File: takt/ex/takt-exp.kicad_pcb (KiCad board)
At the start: 2 copper layers, 40.3 x 128.5 mm, 55 parts, among them J1 PJ301M-12, J2 PJ301M-12, J3 PJ301M-12, J4 PJ301M-12, J5 PJ301M-12, J6 PJ301M-12, J7 PJ301M-12, J8 PJ301M-12, J9 PJ301M-12, Q1 2N3904, Q2 2N3904, Q3 2N3904, SW1 SW_SP3T, SW2 SW_SP3T, SW3 SW_SP3T, U1 TL074, U2 TL074, U3 TL074, U4 ATmega328P-PU

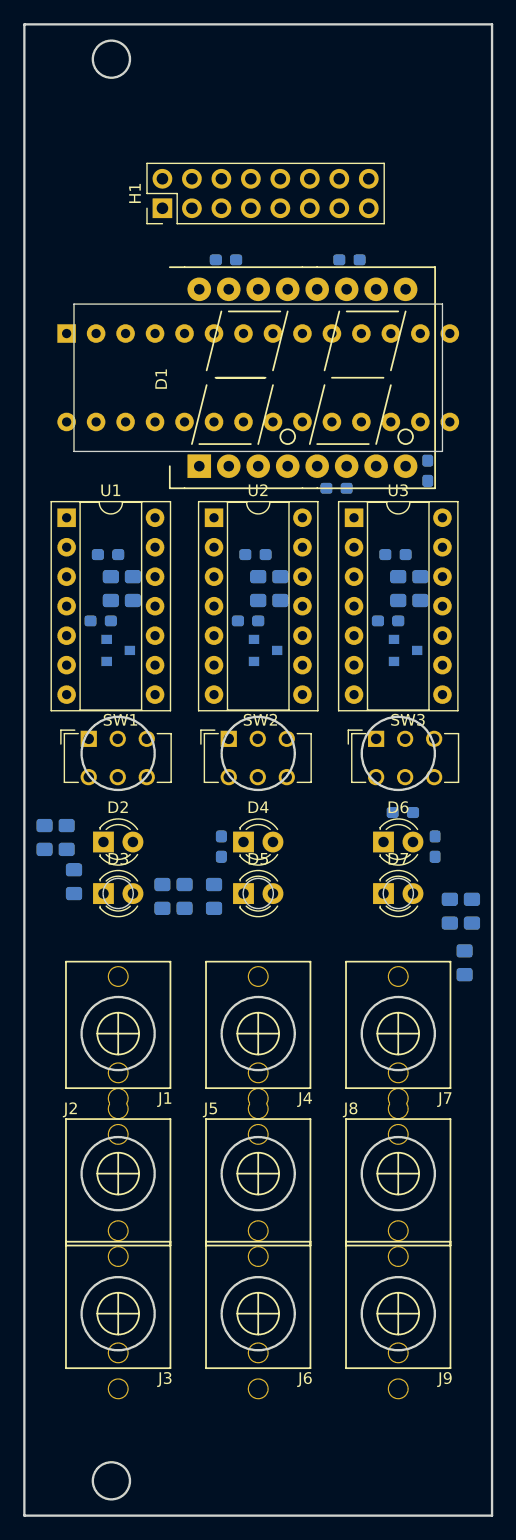
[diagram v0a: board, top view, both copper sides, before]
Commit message: exp traced
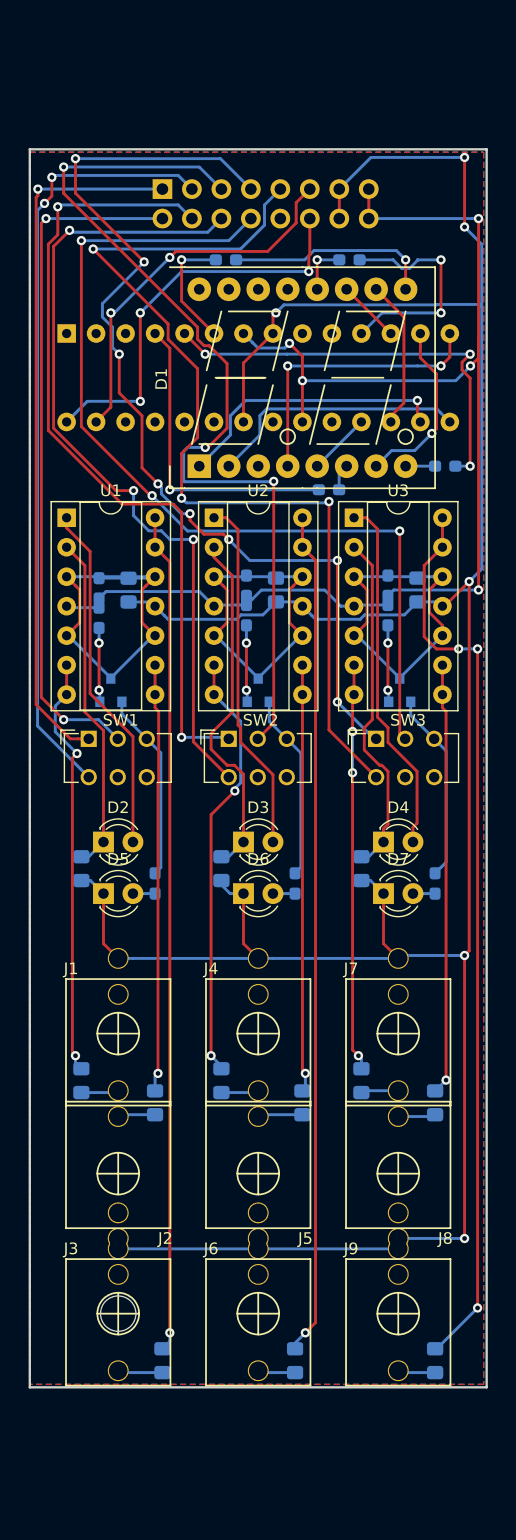
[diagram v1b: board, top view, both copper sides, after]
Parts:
- H1: moved to B.Cu
- moved R7 46.2 mm to (55.2, 143.1)
- moved R10 41.6 mm to (66.7, 143.1)
- moved R13 34.4 mm to (78.7, 143.1)
- moved R24 24.3 mm to (60.3, 100.7)
- moved R25 24.3 mm to (72.4, 100.7)
- moved R23 24.3 mm to (48.3, 100.7)
- moved R6 24.1 mm to (54.6, 120.9)
- moved R9 20.5 mm to (67.3, 120.9)
- moved R11 17.4 mm to (72.4, 119.0)
- moved R5 17.2 mm to (48.3, 119.0)
- moved R12 16.6 mm to (78.7, 120.9)
- moved R8 15.9 mm to (60.3, 119.0)
- moved D6 12.9 mm to (62.2, 102.9)
- moved D3 12.9 mm to (62.2, 98.4)
- moved D4 12.1 mm to (74.3, 98.4)
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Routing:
- net GND: track 0.00 -> 255.8 mm, vias 0 -> 6
- net 5V: track 0.00 -> 113.6 mm, vias 0 -> 5
- net Tr7: track 0.00 -> 85.8 mm, vias 0 -> 8
- net Tr9: track 0.00 -> 83.4 mm, vias 0 -> 3
- net Tr8: track 0.00 -> 80.7 mm, vias 0 -> 3
- net Tr5: track 0.00 -> 80.6 mm, vias 0 -> 3
- net Net-(R13-Pad1): track 0.00 -> 77.8 mm, vias 0 -> 3
- net Net-(R10-Pad1): track 0.00 -> 72.8 mm, vias 0 -> 1
- net Net-(R7-Pad1): track 0.00 -> 72.4 mm, vias 0 -> 1
- net Tr6: track 0.00 -> 70.3 mm, vias 0 -> 3
- net Tr4: track 0.00 -> 69.6 mm, vias 0 -> 2
- net Tr3: track 0.00 -> 66.6 mm, vias 0 -> 2
- net Tr1: track 0.00 -> 61.0 mm, vias 0 -> 1
- net Tr2: track 0.00 -> 59.5 mm, vias 0 -> 2
- net Net-(R12-Pad1): track 0.00 -> 37.2 mm, vias 0 -> 1
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- added copper zone on B.Cu, net GND
- added copper zone on F.Cu, net GND
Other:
- board size 40.3 x 128.5 mm -> 39.4 x 106.7 mm
- board text added: "rot - takt - exp"
